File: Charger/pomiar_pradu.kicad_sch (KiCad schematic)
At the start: 13 parts, among them Q17 IRF7404, Q18 IRF7404, Q19 BC846, U10 MCP6001, U12 ACS712xLCTR-20A, U7 ACS712xLCTR-20A

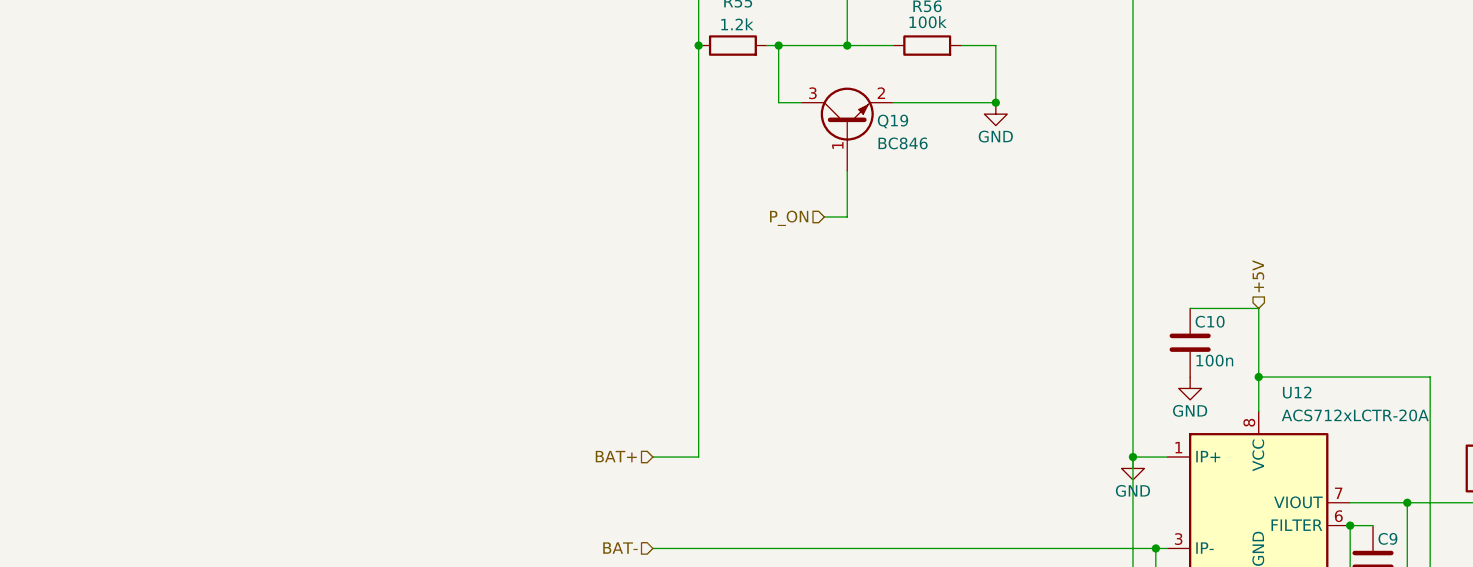
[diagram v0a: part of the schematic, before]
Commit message: poprawki hardware
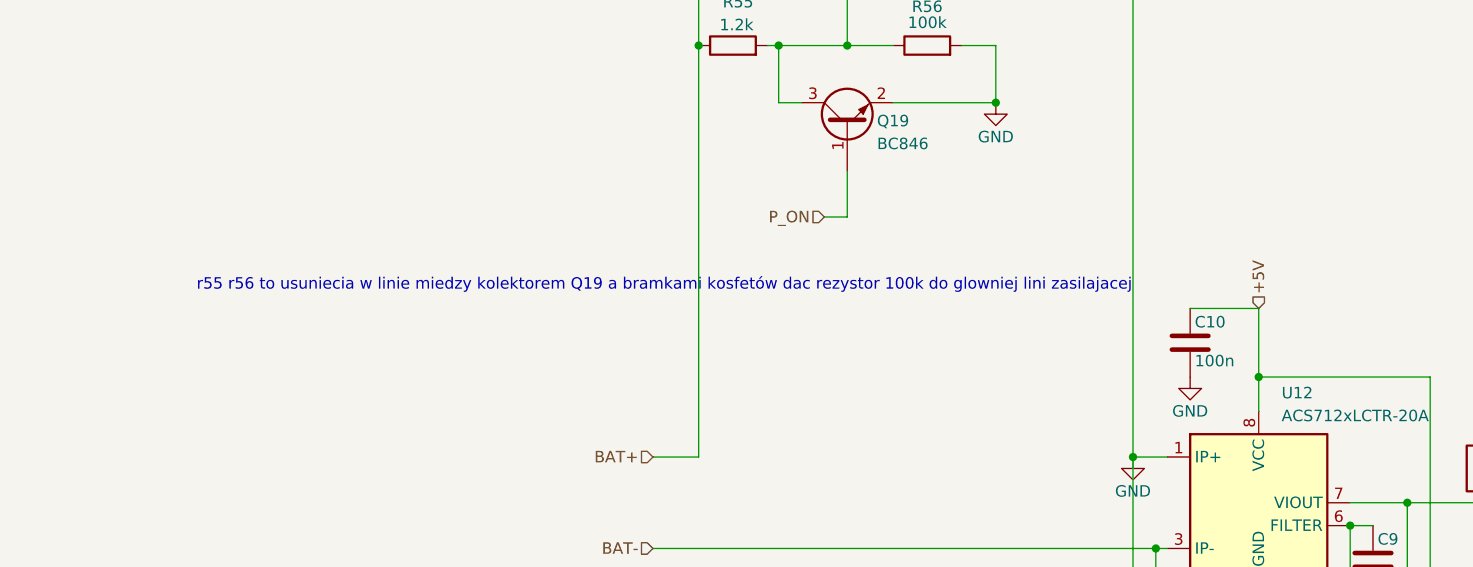
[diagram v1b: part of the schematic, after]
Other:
- note added: "r55 r56 to usuniecia w linie miedzy kolektorem Q19 a bramkami kosfetów dac rezystor 100k do glowniej lini zasilajacej"
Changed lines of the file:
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@@
+		)
+	)
+	(text "r55 r56 to usuniecia w linie miedzy kolektorem Q19 a bramkami kosfetów dac rezystor 100k do glowniej lini zasilajacej "
+		(exclude_from_sim no)
+		(at 83.82 96.52 0)
+		(effects
+			(font
+				(size 1.27 1.27)
+			)
 		)
 	)
